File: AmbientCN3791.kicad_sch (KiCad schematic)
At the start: 56 parts, among them J1 Conn_01x02, J2 Conn_01x02, J3 Conn_01x02, J4 Conn_01x04, J5 Conn_01x04, J7 Conn_01x02, J8 Conn_01x02, Q1 AO3401A, Q2 AO3401A, U1 CN3791, U2 INA3221

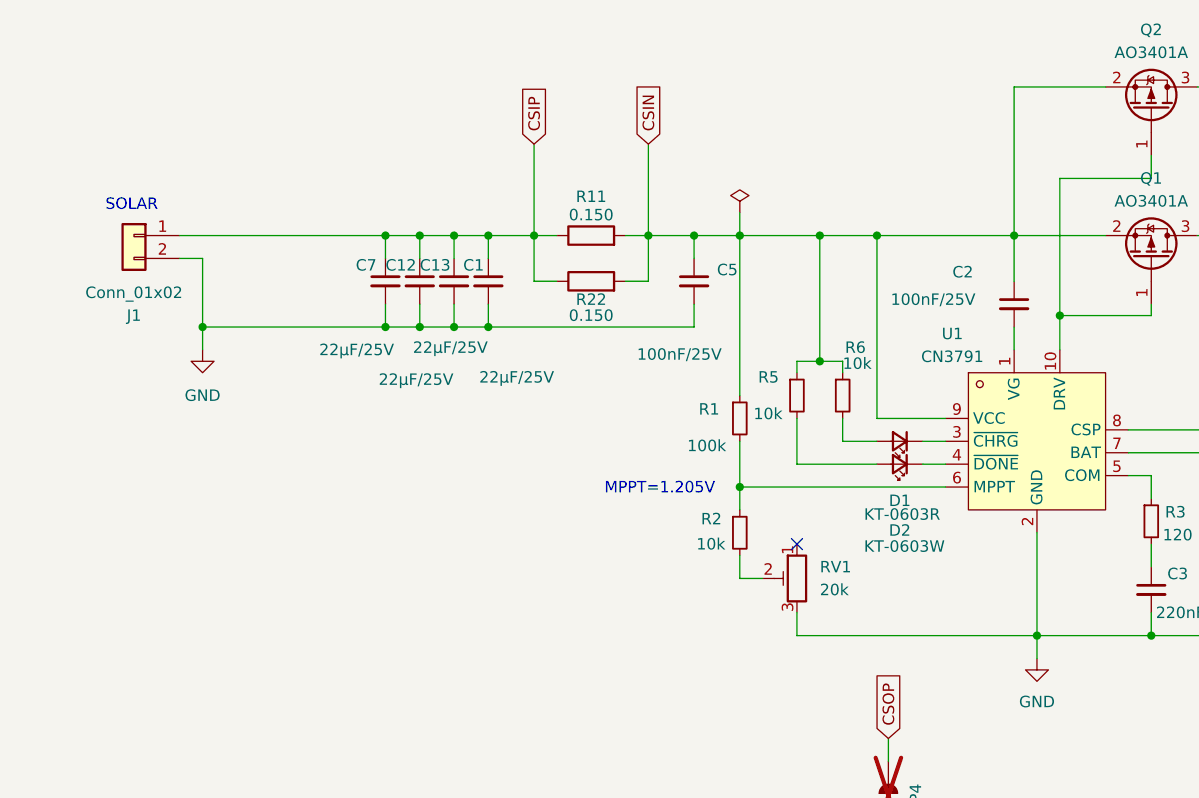
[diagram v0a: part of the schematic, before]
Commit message: WIP2
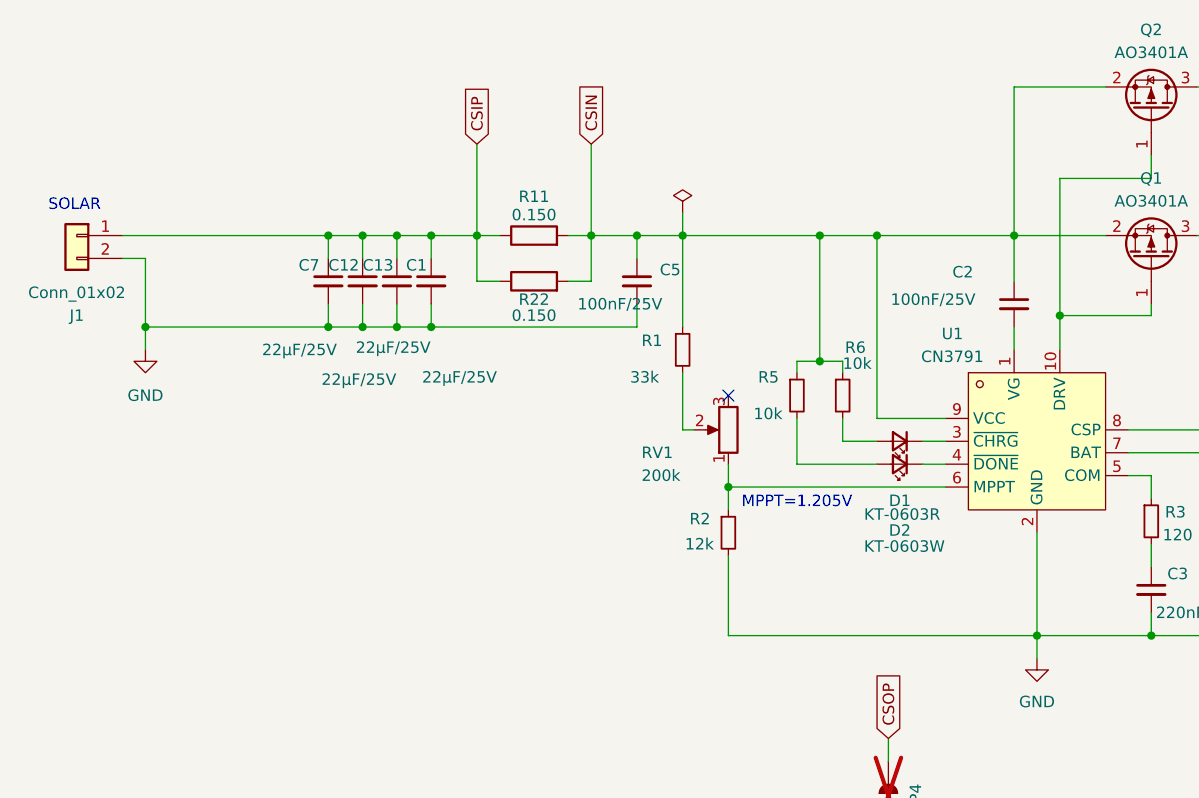
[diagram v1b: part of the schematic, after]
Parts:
- removed RV1: 20k, Potentiometer_SMD:Potentiometer_Bourns_3224J_Horizontal, symbol Device:R_Potentiometer_Trim
- added RV1: 200k, Potentiometer_SMD:Potentiometer_Bourns_3314J_Vertical, symbol Device:R_Potentiometer
- J3: footprint Connector_JST:JST_XH_S2B-XH-A_1x02_P2.50mm_Horizontal -> Connector_PinSocket_2.54mm:PinSocket_1x02_P2.54mm_Vertical
- R1: value 100k -> 33k; LCSC C25741 -> C25779
- R2: value 10k -> 12k; LCSC C25744 -> C25752
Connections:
- net GND: now also R2.2
- net at R2.1, U1.6 (MPPT): now also RV1.1; no longer R1.2
- new net: R1.2, RV1.2
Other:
- moved on the sheet: C1, C12, C13, C5, C7, J1, R1, R11, R2, R22
